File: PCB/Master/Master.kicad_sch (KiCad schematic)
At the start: 72 parts, among them J1 USB_C_Receptacle_USB2.0_16P, J2 Conn_01x05_Pin, J5 Conn_01x09_Pin, J6 Conn_01x09_Pin, Q2 AO3400A, Q3 AO3400A, SW1 PTS810_SJM_250_SMTR_LFS, SW2 PTS810_SJM_250_SMTR_LFS, U1 ESP32-S3-WROOM-1U, U2 TCA9406DC, U3 P82B715D, U4 BME280, U7 SN65HVD230, U9 L5987

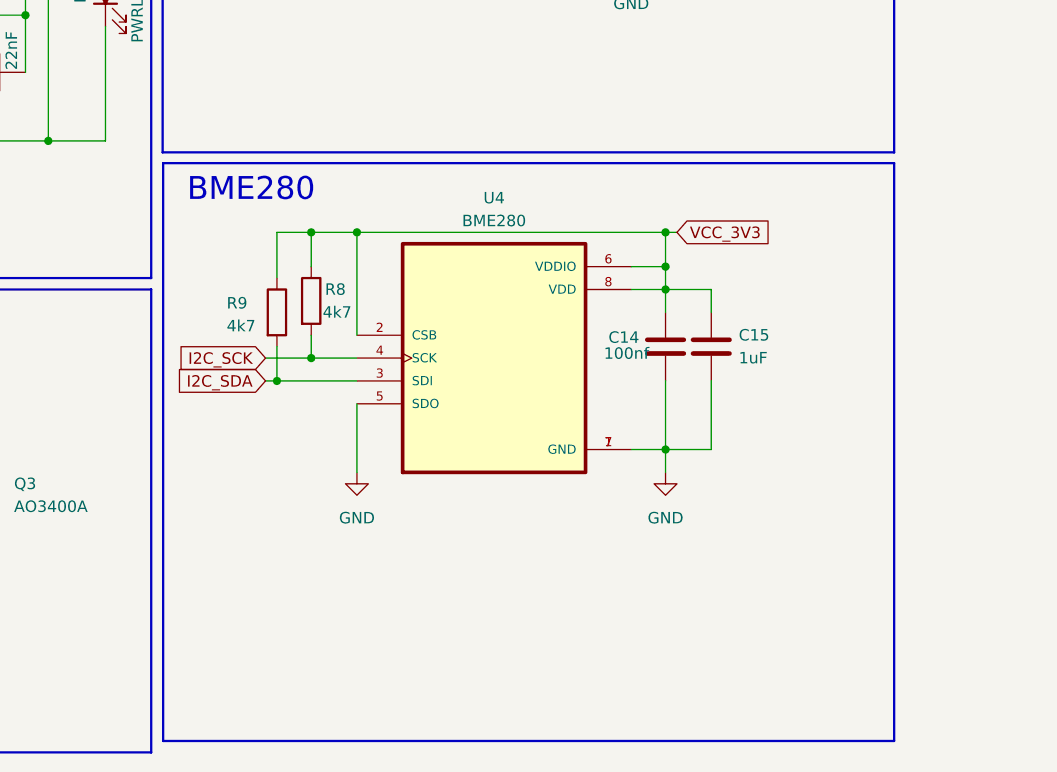
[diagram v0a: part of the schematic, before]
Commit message: Update_Prosinec
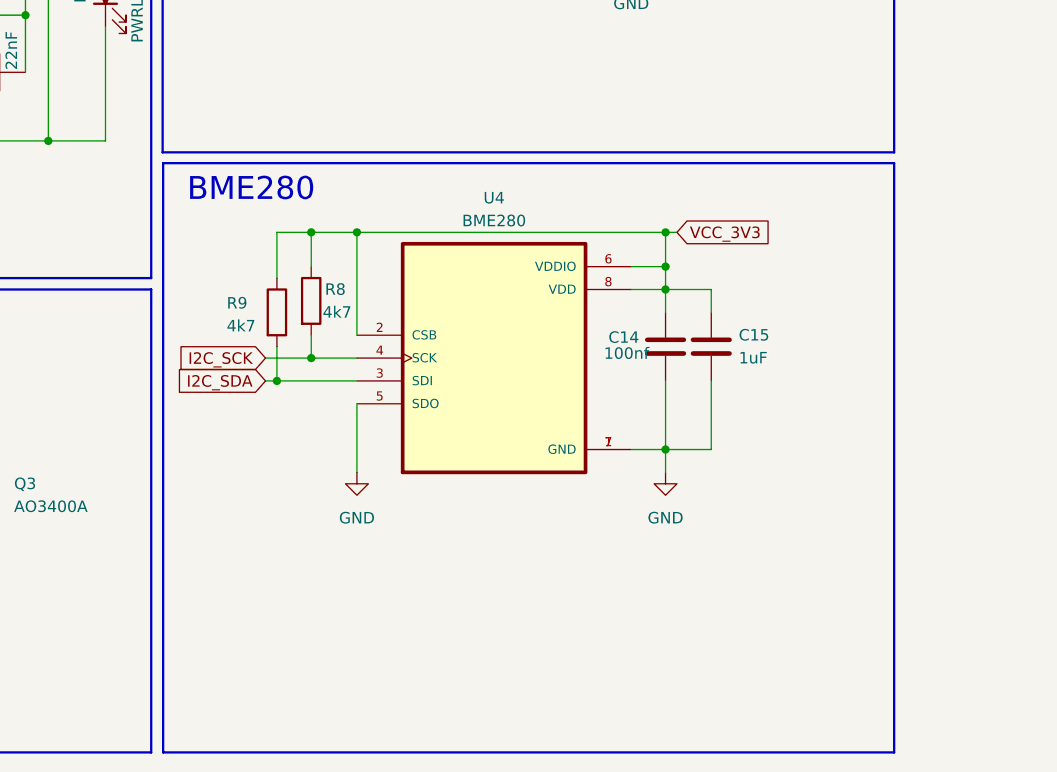
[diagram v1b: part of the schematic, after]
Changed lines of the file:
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@@
 	(rectangle
 		(start 114.3565 119.3101)
-		(end 195.58 183.515)
+		(end 195.58 184.785)
 		(stroke
 			(width 0.254)
